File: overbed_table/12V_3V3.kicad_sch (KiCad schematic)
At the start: 9 parts, among them U2 TPS562201DDCR

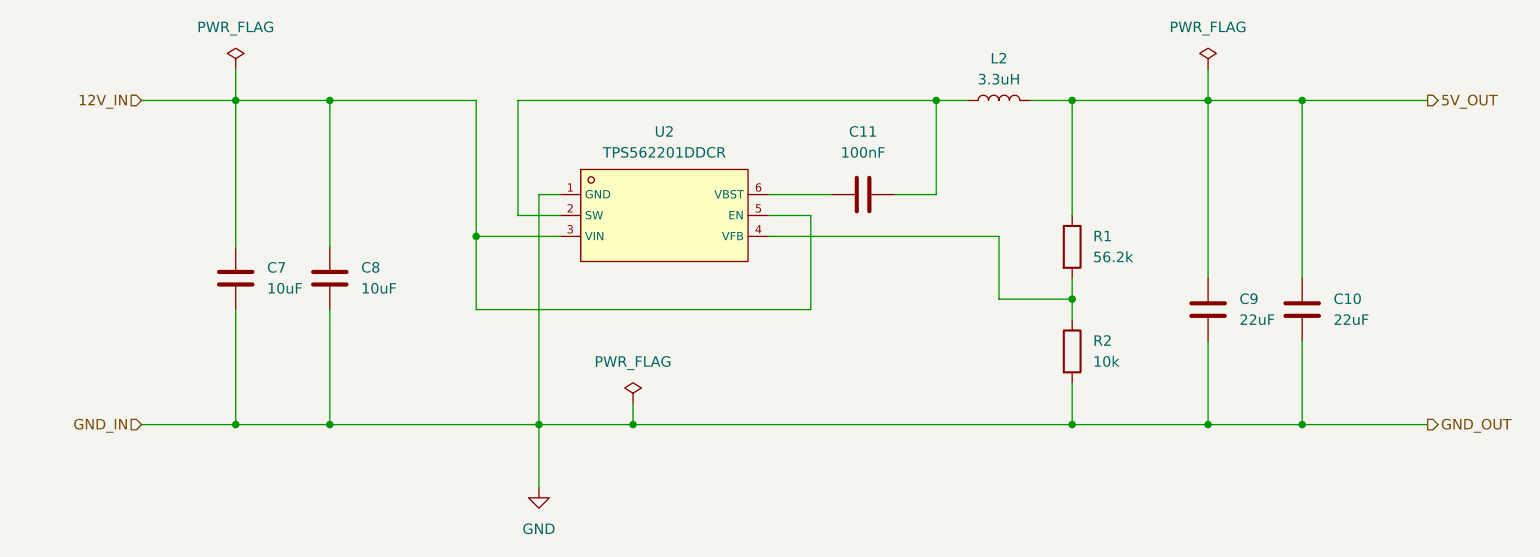
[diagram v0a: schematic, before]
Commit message: 更新12V-5V
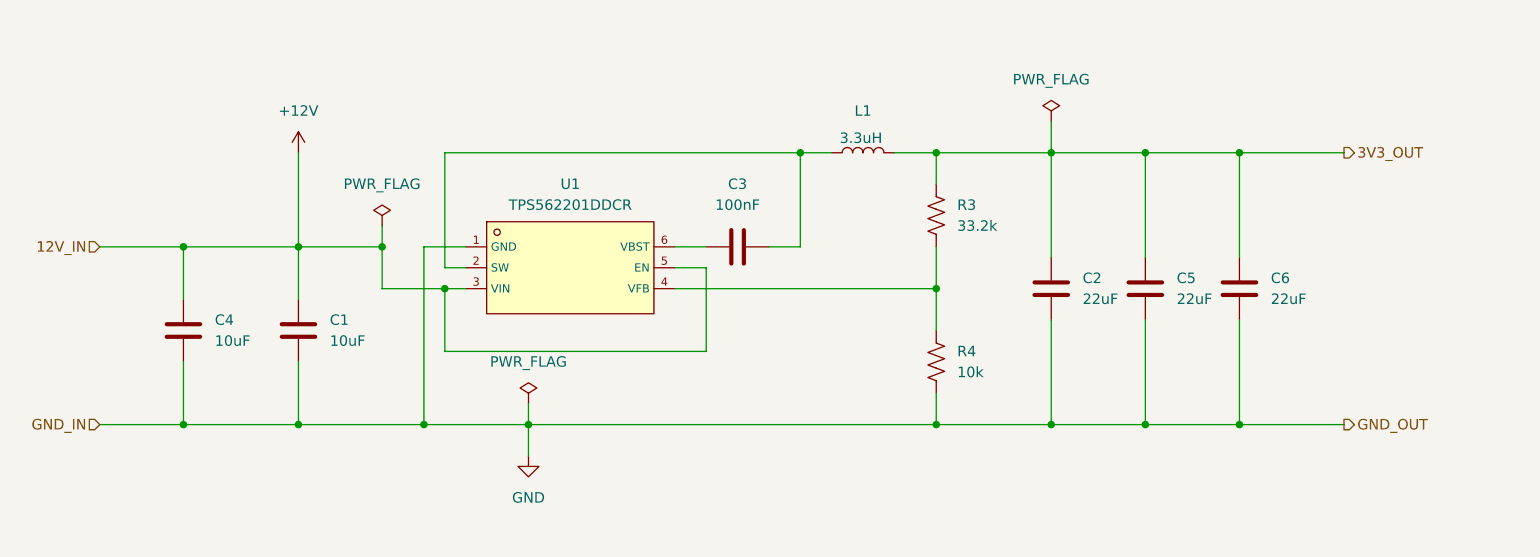
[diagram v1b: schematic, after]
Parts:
- removed C10, C9: 22uF, symbol Device:C
- removed C11: 100nF, symbol Device:C
- removed C7, C8: 10uF, symbol Device:C
- removed L2: 3.3uH, symbol Device:L
- removed R1: 56.2k, lcsc_footprints:C90061_SOT-23-6_L2_9-W1_6-P0_95-LS2_8-BR, symbol Device:R
- removed R2: 10k, symbol Device:R
- removed U2: TPS562201DDCR, lcsc_footprints:C90061_SOT-23-6_L2_9-W1_6-P0_95-LS2_8-BR, symbol lcsc_imported:TPS562201DDCR
- added C1, C4: 10uF, lcsc_footprints:C19188399_SOT-563-6_L1_6-W1_2-P0_50-LS1_6-BL, symbol Device:C
- added C2, C5, C6: 22uF, lcsc_footprints:C19188399_SOT-563-6_L1_6-W1_2-P0_50-LS1_6-BL, symbol Device:C
- added C3: 100nF, lcsc_footprints:C19188399_SOT-563-6_L1_6-W1_2-P0_50-LS1_6-BL, symbol Device:C
- added L1: 3.3uH, symbol Device:L
- added R3: 33.2k, PCM_SparkFun-Resistor:R_0603_1608Metric, symbol PCM_SparkFun-Resistor:R
- added R4: 10k, PCM_SparkFun-Resistor:R_0603_1608Metric, symbol PCM_SparkFun-Resistor:R
- added U1: TPS562201DDCR, lcsc_footprints:C90061_SOT-23-6_L2_9-W1_6-P0_95-LS2_8-BR, symbol lcsc_imported:TPS562201DDCR
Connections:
- net GND: now also C1.2, C2.2, C4.2, C5.2, C6.2, R4.1, U1.1 (GND)
- new net: R3.1, R4.2, U1.4 (VFB)
- new net: C3.2, L1.1, U1.2 (SW)
- new net: C3.1, U1.6 (VBST)
- new net +12V: C1.1, C4.1, U1.3 (VIN), U1.5 (EN)
- new net 3V3_OUT: C2.1, C5.1, C6.1, L1.2, R3.2
